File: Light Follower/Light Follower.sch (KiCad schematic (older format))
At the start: 14 parts, among them P1 Digital, P2 Analog, P3 CONN_01X01, P4 CONN_01X01, P5 CONN_01X01, P6 CONN_01X01

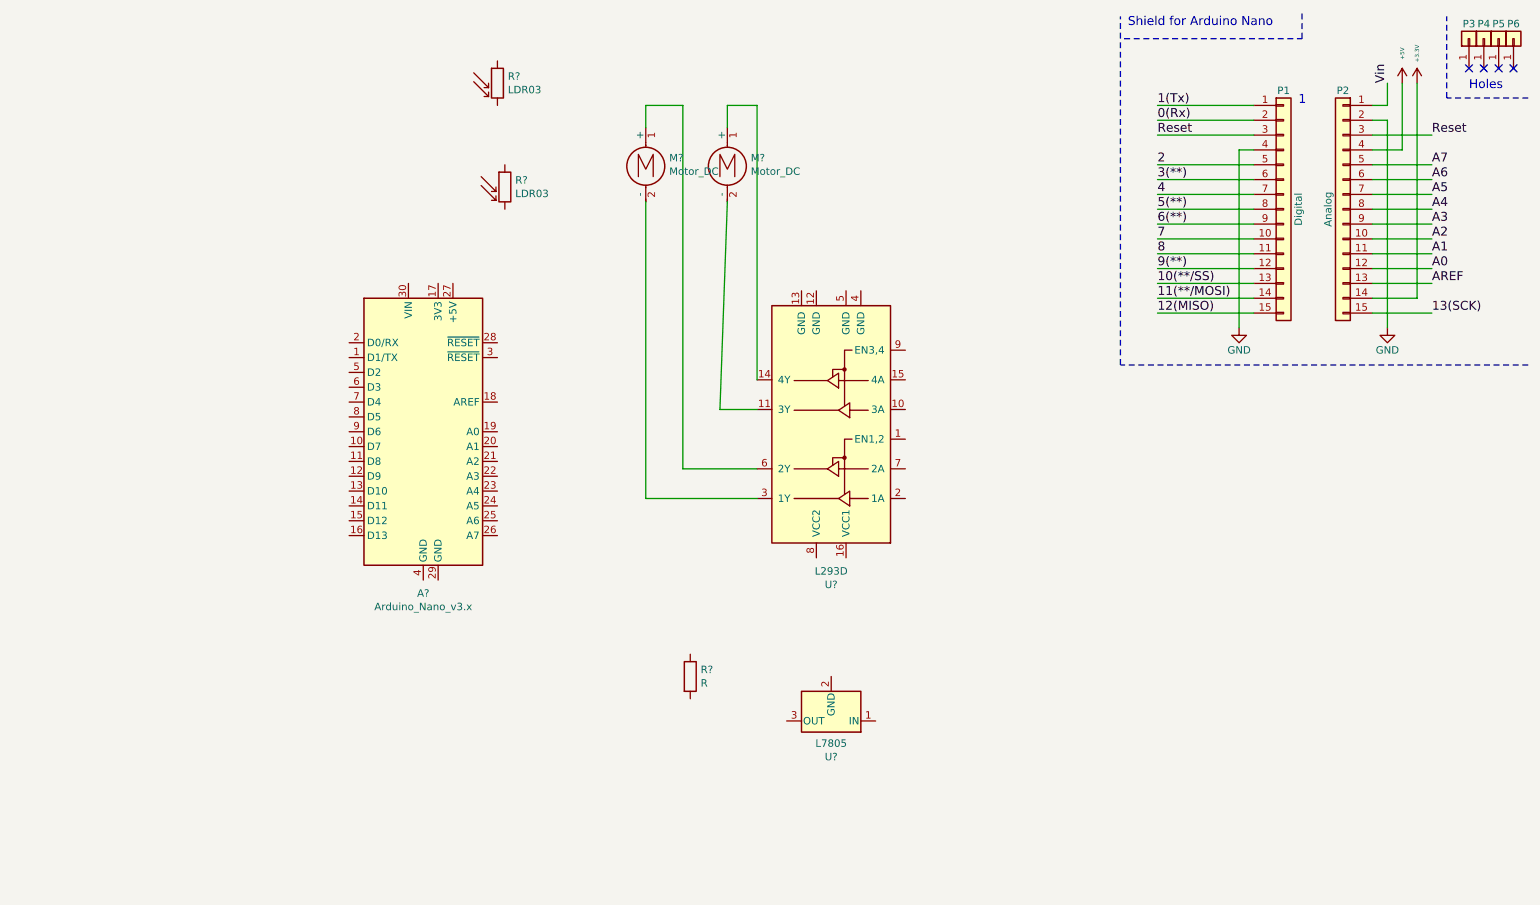
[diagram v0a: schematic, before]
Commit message: Forgot to push the schematic before :')
Manually pushed the folder.
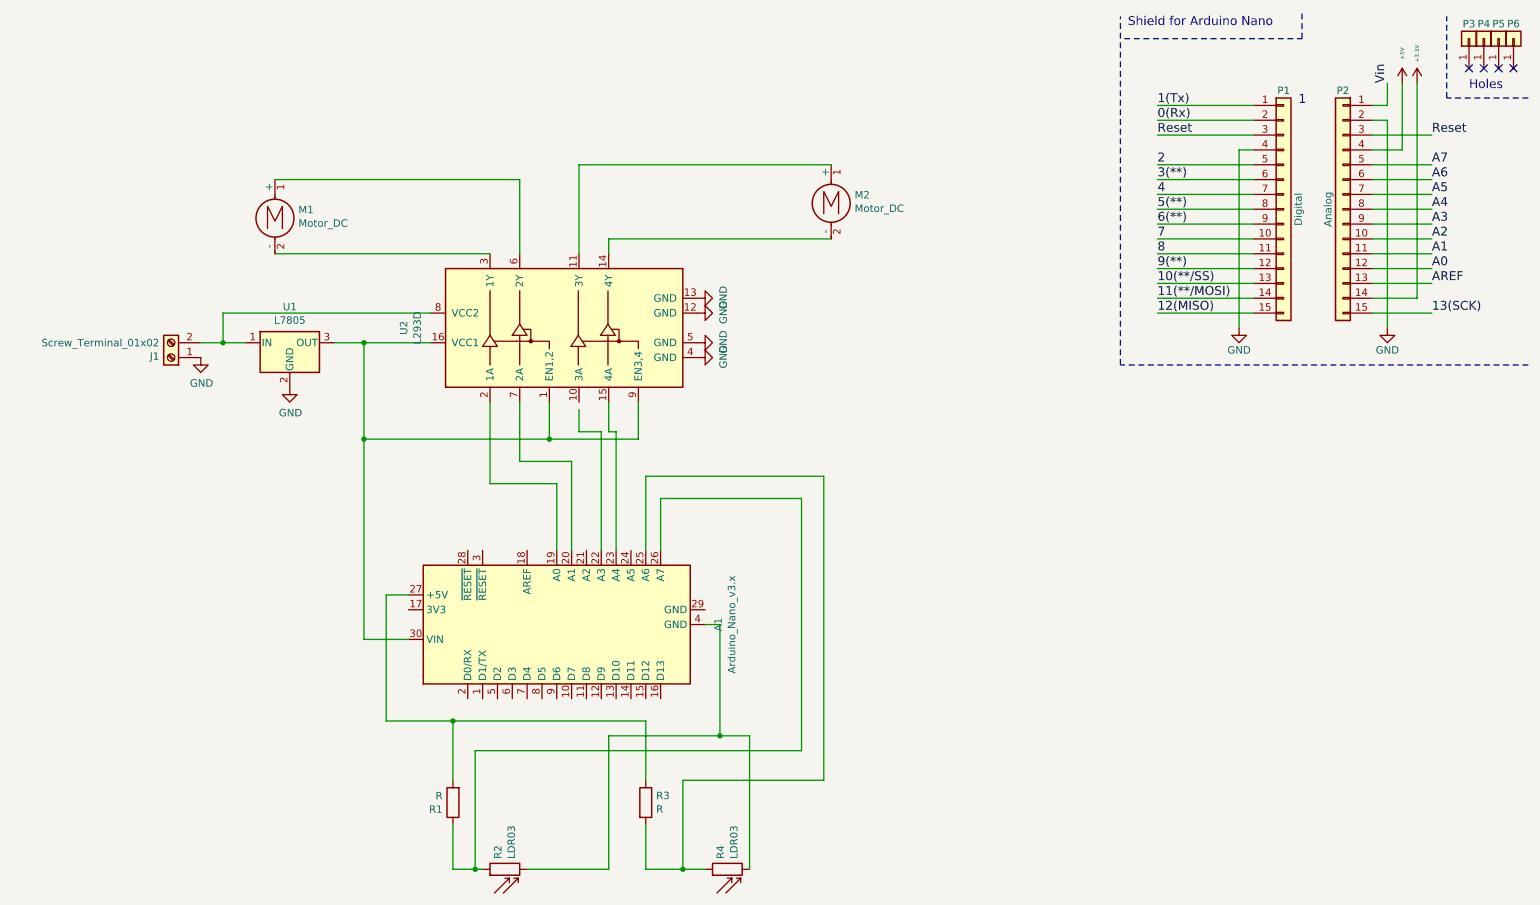
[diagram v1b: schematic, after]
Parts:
- added J1: Screw_Terminal_01x02, symbol Connector:Screw_Terminal_01x02
- added R3: R, symbol Device:R
- gave numbers to parts that had none: 8
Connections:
- net GND: now also U1.2 (GND), U2.12 (GND), U2.13 (GND), U2.4 (GND), U2.5 (GND), J1.1 (Pin_1)
- net at A1.19 (A0): now also U2.2 (1A)
- net at A1.20 (A1): now also U2.7 (2A)
- net at A1.23 (A4): now also U2.15 (4A)
- net at A1.25 (A6): now also R4.1, R3.2
- net at A1.26 (A7): now also R1.1, R2.1
- net at A1.27 (+5V): now also R1.2, R3.1
- net at A1.30 (VIN): now also U1.3 (OUT), U2.1 (EN1,2), U2.16 (VCC1), U2.9 (EN3,4)
- net at A1.4 (GND): now also R2.2, R4.2
- net at M2.1 (+): now also U2.11 (3Y); no longer U2.14 (4Y)
- net at M2.2 (-): now also U2.14 (4Y); no longer U2.11 (3Y)
- net at U2.8 (VCC2): now also U1.1 (IN), J1.2 (Pin_2)
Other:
- moved on the sheet: A1, M1, M2, R1, R2, R4, U1, U2
